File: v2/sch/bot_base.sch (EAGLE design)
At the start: 38 parts, among them K2 DTSM-62K-S-V-T/R, Q0 QWIIC_RIGHT_ANGLE, U1 ESP32-C3-MINI-1-N4, U2 AP7370-33SA (or MCP1703T-3302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, U4 LGS4084HB5

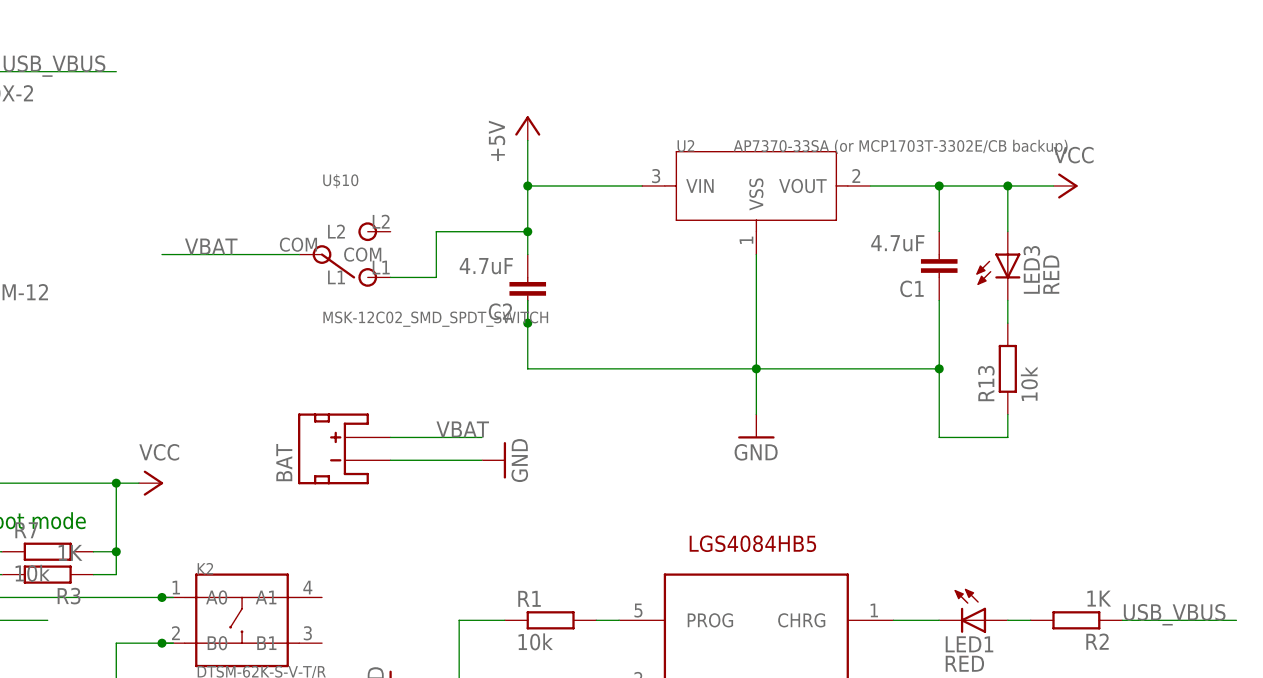
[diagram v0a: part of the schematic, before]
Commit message: latest relayout
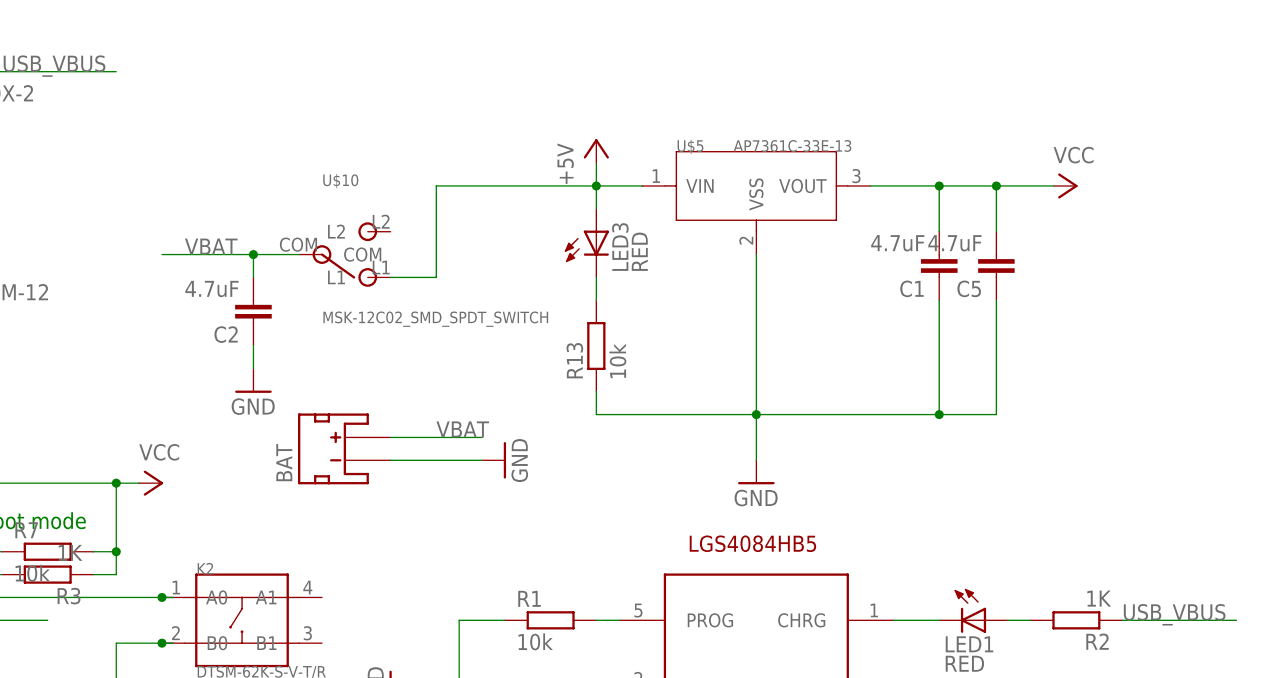
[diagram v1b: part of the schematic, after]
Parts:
- removed U2: AP7370-33SA (or MCP1703T-3302E/CB backup), mcp1703t:MCP1703T
- added C5: 4.7uF, rcl:C-EUC0805
- added U$5: AP7361C-33E-13, vreg:AP7361C-33E-13
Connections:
- net +5V: now also LED3.A, U$5.VIN; no longer C2.2, U2.VIN
- net GND: now also C5.1, U$5.VSS; no longer U2.VSS
- net VBAT: now also C2.2
- net VCC: now also C5.2, U$5.VOUT; no longer LED3.A, U2.VOUT
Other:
- moved on the sheet: C2, LED3, R13
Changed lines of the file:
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@@
 <setting verticaltext="up"/>
 </settings>
-<grid distance="0.1" unitdist="inch" unit="inch" style="lines" multiple="1" display="no" altdistance="0.01" altunitdist="inch" altunit="inch"/>
+<grid distance="0.05" unitdist="inch" unit="inch" style="lines" multiple="1" display="no" altdistance="0.01" altunitdist="inch" altunit="inch"/>
 <layers>
 <layer number="1" name="Top" color="4" fill="1" visible="no" active="no"/>
@@
 <part name="GND10" library="supply1" deviceset="GND" device=""/>
 <part name="P+3" library="supply1" deviceset="VCC" device=""/>
-<part name="U2" library="mcp1703t" deviceset="MCP1703T" device="" value="AP7370-33SA (or MCP1703T-3302E/CB backup)"/>
 <part name="BAT" library="SparkFun-Connectors" deviceset="JST_2MM_MALE" device="" value="C47647 / S2B-PH-SM4-TB"/>
 <part name="GND12" library="supply1" deviceset="GND" device=""/>
@@
 <part name="LED3" library="led" deviceset="LED" device="CHIPLED_0603" value="RED"/>
 <part name="R13" library="rcl" deviceset="R-EU_" device="R0603" value="10k"/>
+<part name="GND14" library="supply1" deviceset="GND" device=""/>
+<part name="U$5" library="vreg" deviceset="AP7361C-33E-13" device=""/>
+<part name="C5" library="rcl" deviceset="C-EU" device="C0805" value="4.7uF"/>
 </parts>
 <sheets>
@@
 <instance part="LED1" gate="G$1" x="172.72" y="83.82" rot="R270"/>
 <instance part="C1" gate="G$1" x="167.64" y="121.92" rot="R180"/>
-<instance part="GND10" gate="1" x="147.32" y="104.14"/>
+<instance part="GND10" gate="1" x="147.32" y="99.06"/>
 <instance part="P+3" gate="VCC" x="182.88" y="132.08" rot="R270"/>
-<instance part="U2" gate="G$1" x="147.32" y="132.08"/>
 <instance part="BAT" gate="G$1" x="101.6" y="101.6" rot="R90"/>
 <instance part="GND12" gate="1" x="119.38" y="101.6" rot="R90"/>
-<instance part="C2" gate="G$1" x="121.92" y="119.38" rot="R180"/>
+<instance part="C2" gate="G$1" x="91.44" y="116.84" rot="R180"/>
 <instance part="C3" gate="G$1" x="38.1" y="-20.32" rot="R180"/>
 <instance part="C4" gate="G$1" x="38.1" y="5.08" rot="R180"/>
-<instance part="P+1" gate="1" x="121.92" y="139.7"/>
+<instance part="P+1" gate="1" x="129.54" y="137.16"/>
 <instance part="P+2" gate="1" x="38.1" y="17.78"/>
 <instance part="P+4" gate="1" x="38.1" y="-7.62"/>
@@
 <instance part="K2" gate="G$1" x="90.17" y="83.82"/>
 <instance part="U$10" gate="MSK-12C02" x="104.14" y="124.46"/>
-<instance part="LED3" gate="G$1" x="175.26" y="124.46"/>
-<instance part="R13" gate="G$1" x="175.26" y="111.76" rot="R90"/>
+<instance part="LED3" gate="G$1" x="129.54" y="127"/>
+<instance part="R13" gate="G$1" x="129.54" y="114.3" rot="R90"/>
+<instance part="GND14" gate="1" x="91.44" y="109.22"/>
+<instance part="U$5" gate="G$1" x="147.32" y="132.08"/>
+<instance part="C5" gate="G$1" x="173.99" y="121.92" rot="R180"/>
 </instances>
 <busses>
@@
 </segment>
 <segment>
-<pinref part="GND10" gate="1" pin="GND"/>
-<wire x1="147.32" y1="111.76" x2="147.32" y2="106.68" width="0.1524" layer="91"/>
-<wire x1="121.92" y1="111.76" x2="147.32" y2="111.76" width="0.1524" layer="91"/>
-<pinref part="C1" gate="G$1" pin="1"/>
-<wire x1="147.32" y1="111.76" x2="167.64" y2="111.76" width="0.1524" layer="91"/>
-<wire x1="167.64" y1="111.76" x2="167.64" y2="119.38" width="0.1524" layer="91"/>
-<junction x="147.32" y="111.76"/>
-<wire x1="147.32" y1="124.46" x2="147.32" y2="111.76" width="0.1524" layer="91"/>
-<pinref part="U2" gate="G$1" pin="VSS"/>
-<wire x1="121.92" y1="119.38" x2="121.92" y2="116.84" width="0.1524" layer="91"/>
-<pinref part="C2" gate="G$1" pin="1"/>
-<wire x1="121.92" y1="116.84" x2="121.92" y2="111.76" width="0.1524" layer="91"/>
-<junction x="121.92" y="116.84"/>
-<pinref part="R13" gate="G$1" pin="1"/>
-<wire x1="175.26" y1="106.68" x2="175.26" y2="104.14" width="0.1524" layer="91"/>
-<wire x1="175.26" y1="104.14" x2="167.64" y2="104.14" width="0.1524" layer="91"/>
-<wire x1="167.64" y1="104.14" x2="167.64" y2="111.76" width="0.1524" layer="91"/>
-<junction x="167.64" y="111.76"/>
-</segment>
-<segment>
 <pinref part="BAT" gate="G$1" pin="-"/>
 <pinref part="GND12" gate="1" pin="GND"/>
@@
 <pinref part="GND13" gate="1" pin="GND"/>
 </segment>
+<segment>
+<wire x1="91.44" y1="111.76" x2="91.44" y2="114.3" width="0.1524" layer="91"/>
+<pinref part="C2" gate="G$1" pin="1"/>
+<pinref part="GND14" gate="1" pin="GND"/>
+</segment>
+<segment>
+<pinref part="GND10" gate="1" pin="GND"/>
+<wire x1="147.32" y1="106.68" x2="147.32" y2="101.6" width="0.1524" layer="91"/>
+<pinref part="C1" gate="G$1" pin="1"/>
+<wire x1="129.54" y1="106.68" x2="147.32" y2="106.68" width="0.1524" layer="91"/>
+<wire x1="147.32" y1="106.68" x2="167.64" y2="106.68" width="0.1524" layer="91"/>
+<wire x1="167.64" y1="106.68" x2="167.64" y2="119.38" width="0.1524" layer="91"/>
+<junction x="147.32" y="106.68"/>
+<wire x1="147.32" y1="124.46" x2="147.32" y2="106.68" width="0.1524" layer="91"/>
+<pinref part="R13" gate="G$1" pin="1"/>
+<wire x1="129.54" y1="109.22" x2="129.54" y2="106.68" width="0.1524" layer="91"/>
+<pinref part="U$5" gate="G$1" pin="VSS"/>
+<pinref part="C5" gate="G$1" pin="1"/>
+<wire x1="173.99" y1="119.38" x2="173.99" y2="106.68" width="0.1524" layer="91"/>
+<wire x1="173.99" y1="106.68" x2="167.64" y2="106.68" width="0.1524" layer="91"/>
+<junction x="167.64" y="106.68"/>
+</segment>
 </net>
 <net name="MOTOR1A" class="0">
@@
 <label x="83.82" y="124.46" size="1.778" layer="95"/>
 <pinref part="U$10" gate="MSK-12C02" pin="COM"/>
-<wire x1="81.28" y1="124.46" x2="96.52" y2="124.46" width="0.1524" layer="91"/>
+<wire x1="81.28" y1="124.46" x2="91.44" y2="124.46" width="0.1524" layer="91"/>
+<pinref part="C2" gate="G$1" pin="2"/>
+<wire x1="91.44" y1="124.46" x2="96.52" y2="124.46" width="0.1524" layer="91"/>
+<wire x1="91.44" y1="121.92" x2="91.44" y2="124.46" width="0.1524" layer="91"/>
+<junction x="91.44" y="124.46"/>
 </segment>
 </net>
@@
 <pinref part="P+3" gate="VCC" pin="VCC"/>
 <pinref part="C1" gate="G$1" pin="2"/>
-<wire x1="167.64" y1="132.08" x2="175.26" y2="132.08" width="0.1524" layer="91"/>
-<wire x1="175.26" y1="132.08" x2="180.34" y2="132.08" width="0.1524" layer="91"/>
+<wire x1="167.64" y1="132.08" x2="173.99" y2="132.08" width="0.1524" layer="91"/>
+<wire x1="173.99" y1="132.08" x2="180.34" y2="132.08" width="0.1524" layer="91"/>
 <wire x1="167.64" y1="127" x2="167.64" y2="132.08" width="0.1524" layer="91"/>
 <junction x="167.64" y="132.08"/>
-<pinref part="U2" gate="G$1" pin="VOUT"/>
 <wire x1="167.64" y1="132.08" x2="160.02" y2="132.08" width="0.1524" layer="91"/>
-<pinref part="LED3" gate="G$1" pin="A"/>
-<wire x1="175.26" y1="132.08" x2="175.26" y2="127" width="0.1524" layer="91"/>
-<junction x="175.26" y="132.08"/>
+<pinref part="U$5" gate="G$1" pin="VOUT"/>
+<pinref part="C5" gate="G$1" pin="2"/>
+<wire x1="173.99" y1="132.08" x2="173.99" y2="127" width="0.1524" layer="91"/>
+<junction x="173.99" y="132.08"/>
 </segment>
 <segment>
@@
 <net name="+5V" class="0">
 <segment>
-<wire x1="134.62" y1="132.08" x2="121.92" y2="132.08" width="0.1524" layer="91"/>
-<wire x1="121.92" y1="132.08" x2="121.92" y2="137.16" width="0.1524" layer="91"/>
-<pinref part="U2" gate="G$1" pin="VIN"/>
-<junction x="121.92" y="132.08"/>
-<wire x1="121.92" y1="124.46" x2="121.92" y2="127" width="0.1524" layer="91"/>
-<wire x1="121.92" y1="127" x2="121.92" y2="132.08" width="0.1524" layer="91"/>
-<junction x="121.92" y="127"/>
-<pinref part="C2" gate="G$1" pin="2"/>
+<wire x1="134.62" y1="132.08" x2="129.54" y2="132.08" width="0.1524" layer="91"/>
+<wire x1="129.54" y1="132.08" x2="129.54" y2="134.62" width="0.1524" layer="91"/>
+<junction x="129.54" y="132.08"/>
 <pinref part="P+1" gate="1" pin="+5V"/>
 <pinref part="U$10" gate="MSK-12C02" pin="L1"/>
-<wire x1="111.76" y1="127" x2="121.92" y2="127" width="0.1524" layer="91"/>
+<wire x1="111.76" y1="132.08" x2="129.54" y2="132.08" width="0.1524" layer="91"/>
 <wire x1="106.68" y1="121.92" x2="111.76" y2="121.92" width="0.1524" layer="91"/>
-<wire x1="111.76" y1="121.92" x2="111.76" y2="127" width="0.1524" layer="91"/>
+<wire x1="111.76" y1="121.92" x2="111.76" y2="132.08" width="0.1524" layer="91"/>
+<pinref part="LED3" gate="G$1" pin="A"/>
+<wire x1="129.54" y1="129.54" x2="129.54" y2="132.08" width="0.1524" layer="91"/>
+<pinref part="U$5" gate="G$1" pin="VIN"/>
 </segment>
 <segment>
@@
 <pinref part="LED3" gate="G$1" pin="C"/>
 <pinref part="R13" gate="G$1" pin="2"/>
-<wire x1="175.26" y1="119.38" x2="175.26" y2="116.84" width="0.1524" layer="91"/>
-</segment>
-</net>
+<wire x1="129.54" y1="121.92" x2="129.54" y2="119.38" width="0.1524" layer="91"/>
+</segment>
+</net>
